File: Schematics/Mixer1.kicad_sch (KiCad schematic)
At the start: 47 parts, among them J70 Conn_01x02, J71 Conn_01x02, J72 Conn_01x02, J73 AudioJack2_Ground, J74 Conn_01x02, J75 Conn_01x02, J76 Conn_01x02, J77 Conn_01x02, J78 Conn_01x02, J79 Conn_01x02, J80 Conn_01x03, U101 LM358, U119 TL084, U120 LM358, U121 TL084

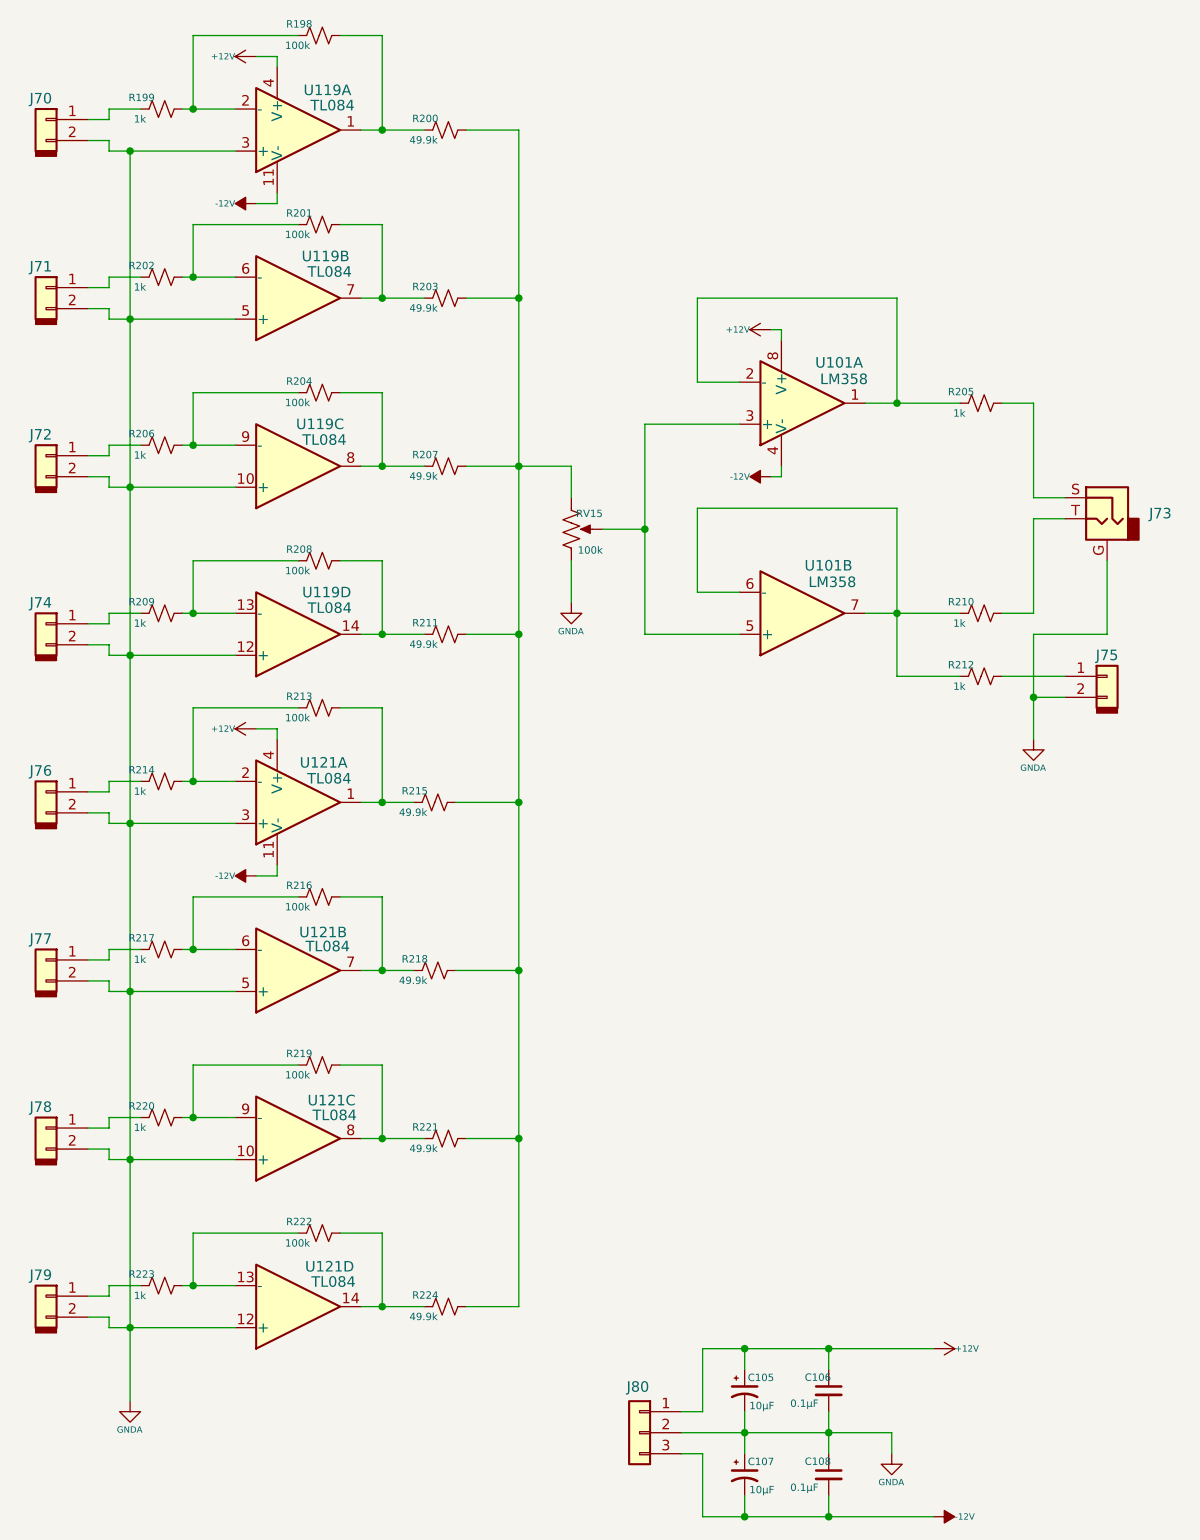
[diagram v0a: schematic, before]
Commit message: updated schematics.
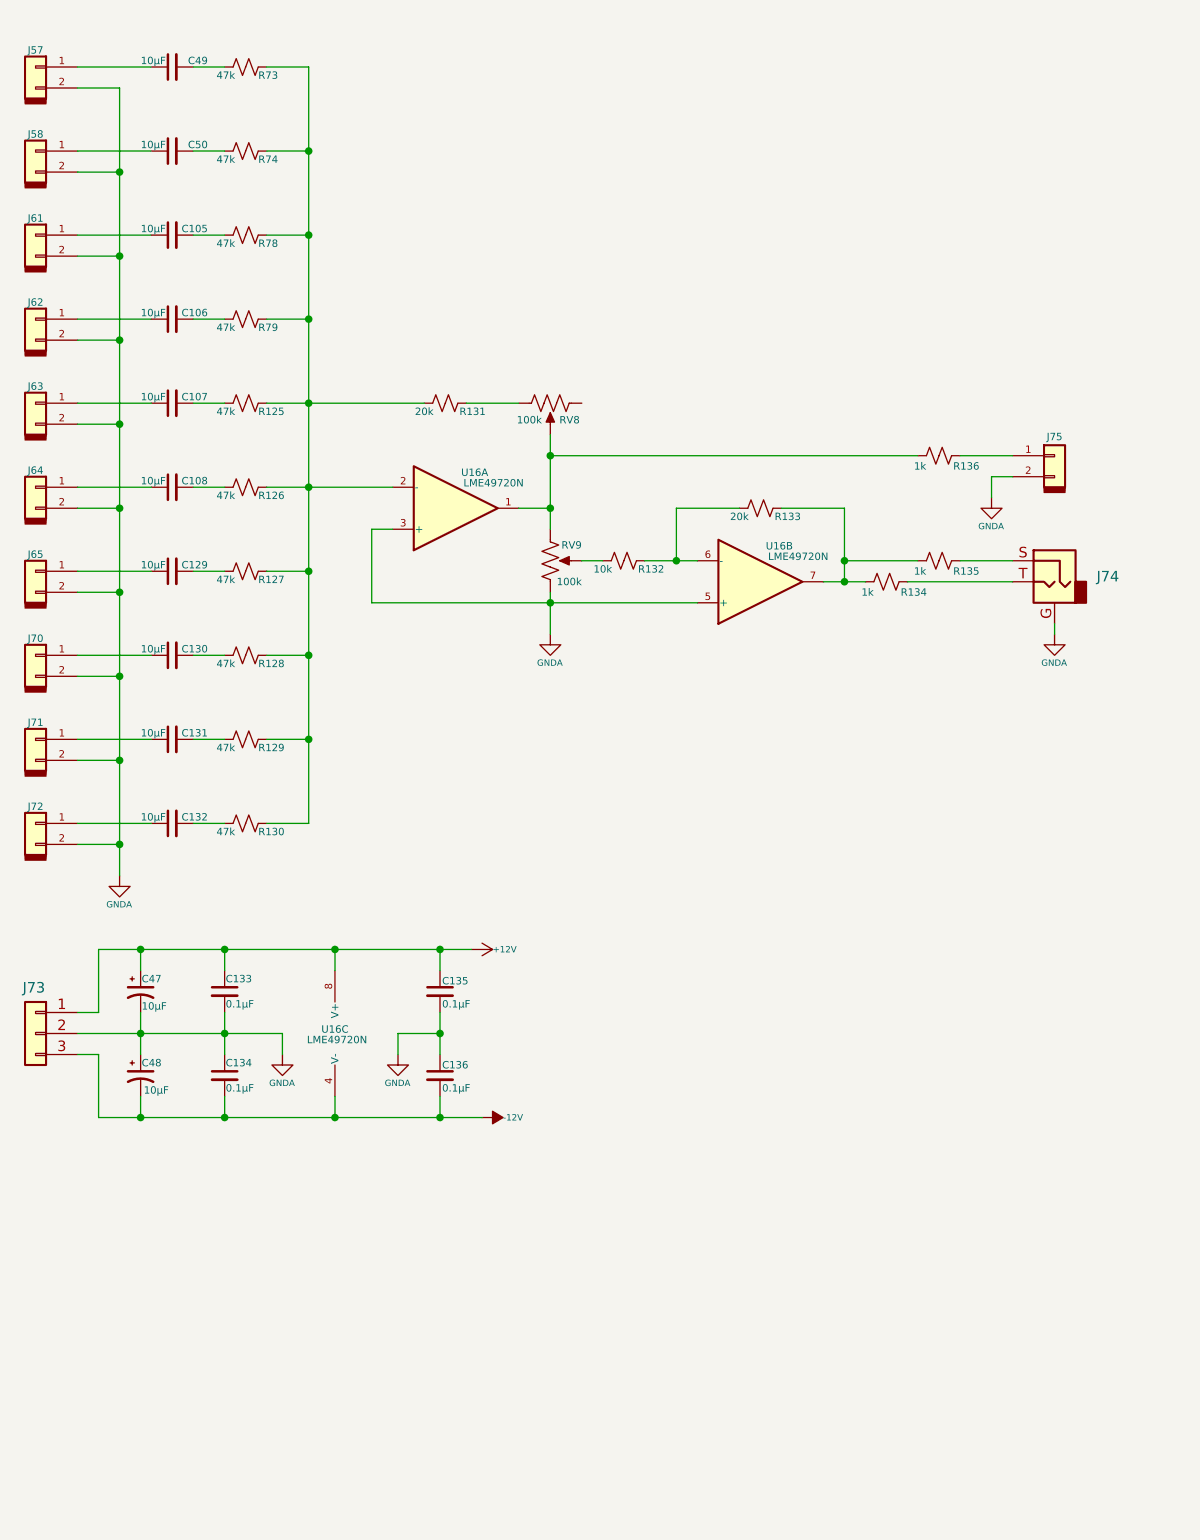
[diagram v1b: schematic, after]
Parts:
- removed J74, J76, J77, J78, J79: Conn_01x02, symbol Connector_keyed_kicad_sym:Conn_01x02
- removed R198, R201, R204, R208, R213, R216, R219, R222: 100k, symbol Device:R_Small_US
- removed R199, R202, R205, R206, R209, R212, R214, R217, R220, R223: 1k, symbol Device:R_Small_US
- removed R200, R203, R207, R211, R215, R218, R221, R224: 49.9k, symbol Device:R_Small_US
- removed U101, U120: LM358, symbol Amplifier_Operational:LM358
- removed U119, U121: TL084, symbol Amplifier_Operational:TL084
- added C105, C106, C107, C108, C129, C130, C131, C132, C49, C50: 10µF, symbol Device:C_Small
- added C135, C136: 0.1µF, symbol Device:C_Small
- added J57, J58, J61, J63, J64, J65, J72: Conn_01x02, symbol Connector_keyed_kicad_sym:Conn_01x02
- added R125, R126, R127, R128, R129, R130, R73, R74, R78, R79: 47k, symbol Device:R_Small_US
- added R131, R133: 20k, symbol Device:R_Small_US
- added R132: 10k, symbol Device:R_Small_US
- added R135, R136: 1k, symbol Device:R_Small_US
- added RV8: 100k, symbol Device:R_Potentiometer_US
- added U16: LME49720N, symbol Amplifier_Operational:TL072
- renumbered C106 to C133, C108 to C134, C105 to C47, C107 to C48, J72 to J62, J80 to J73, J73 to J74, R210 to R134, RV15 to RV9
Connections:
- net +12V: now also C135.1, U16.8 (V+)
- net -12V: now also C136.2, U16.4 (V-)
- net GNDA: now also C135.2, C136.1, J57.2 (Pin_2), J58.2 (Pin_2), J61.2 (Pin_2), J63.2 (Pin_2), J64.2 (Pin_2), J65.2 (Pin_2), J72.2 (Pin_2), U16.3 (+), U16.5 (+)
- net at R134.1: now also R133.2, R135.1, U16.7
- net at J75.1 (Pin_1): now also R136.2
- net at J62.1 (Pin_1): now also C106.1
- net at J74.S: now also R135.2
- net at J70.1 (Pin_1): now also C130.1
- net at J71.1 (Pin_1): now also C131.1
- new net: C49.2, R73.1
- new net: R125.2, R126.2, R127.2, R128.2, R129.2, R130.2, R131.1, R73.2, R74.2, R78.2, R79.2, U16.2 (-)
- new net: C130.2, R128.1
- new net: C106.2, R79.1
- new net: C107.1, J63.1 (Pin_1)
- new net: C107.2, R125.1
- new net: C49.1, J57.1 (Pin_1)
- new net: C132.2, R130.1
- new net: C132.1, J72.1 (Pin_1)
- new net: R136.1, RV8. (3), RV9. (3), U16.1
- new net: R132.1, RV9. (3)
- new net: R132.2, R133.1, U16.6 (-)
- new net: C129.1, J65.1 (Pin_1)
- new net: C129.2, R127.1
- new net: C105.2, R78.1
- new net: R131.2, RV8. (3)
- new net: C50.2, R74.1
- new net: C105.1, J61.1 (Pin_1)
- new net: C50.1, J58.1 (Pin_1)
- new net: C108.2, R126.1
- new net: C131.2, R129.1
- new net: C108.1, J64.1 (Pin_1)
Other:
- moved on the sheet: C133, C134, C47, C48, J62, J73, J74, J75, R134, RV9
